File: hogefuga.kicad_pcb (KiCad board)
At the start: 2 copper layers, 95.3 x 97.6 mm, 45 parts, among them J1 MJ-4PP-9, SW1 SW_PUSH, SW10 SW_PUSH, SW11 SW_PUSH, SW12 SW_PUSH, SW13 SW_PUSH, SW14 SW_PUSH, SW15 SW_PUSH, SW16 SW_PUSH, SW17 SW_PUSH, SW18 SW_PUSH, SW19 SW_PUSH, SW2 SW_PUSH, SW20 SW_PUSH, SW3 SW_PUSH, SW4 SW_PUSH, SW5 SW_PUSH, SW6 SW_PUSH, SW7 SW_PUSH, SW8 SW_PUSH, SW9 SW_PUSH, U1 ProMicro

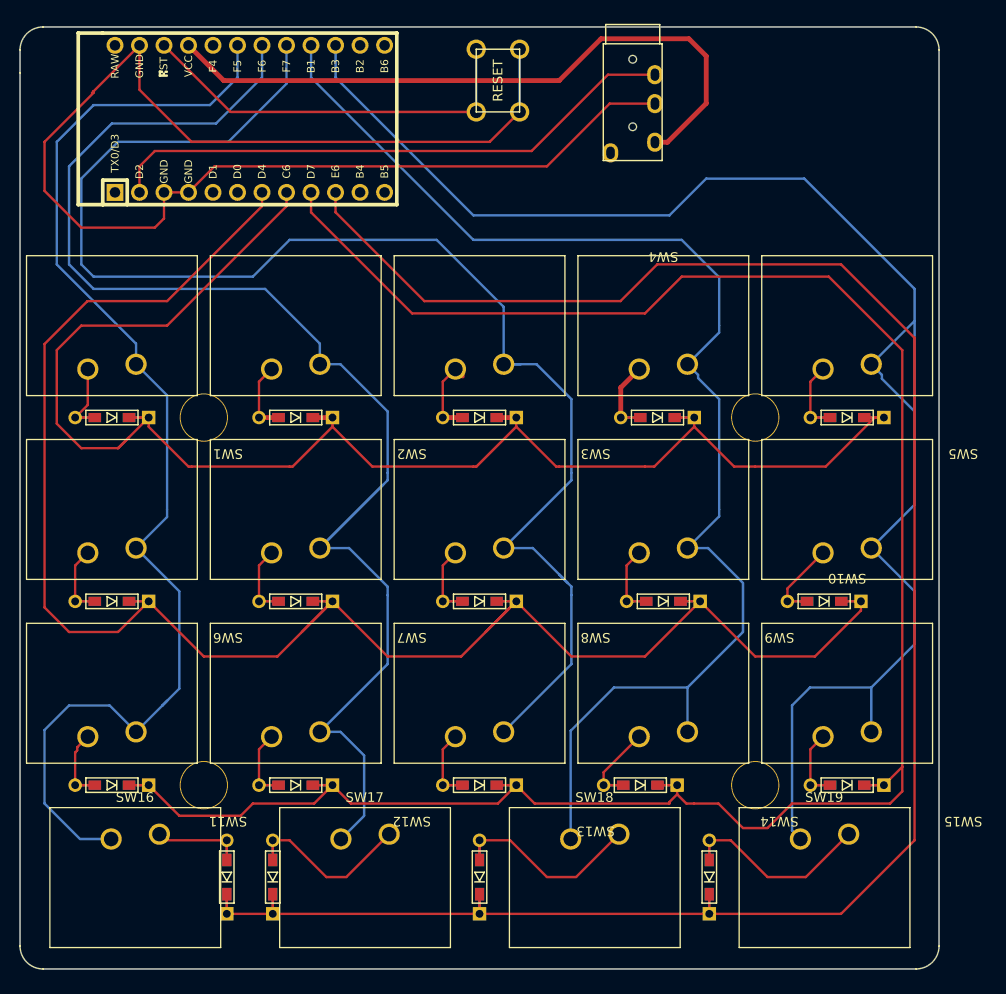
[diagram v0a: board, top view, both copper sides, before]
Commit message: GND塗りつぶし
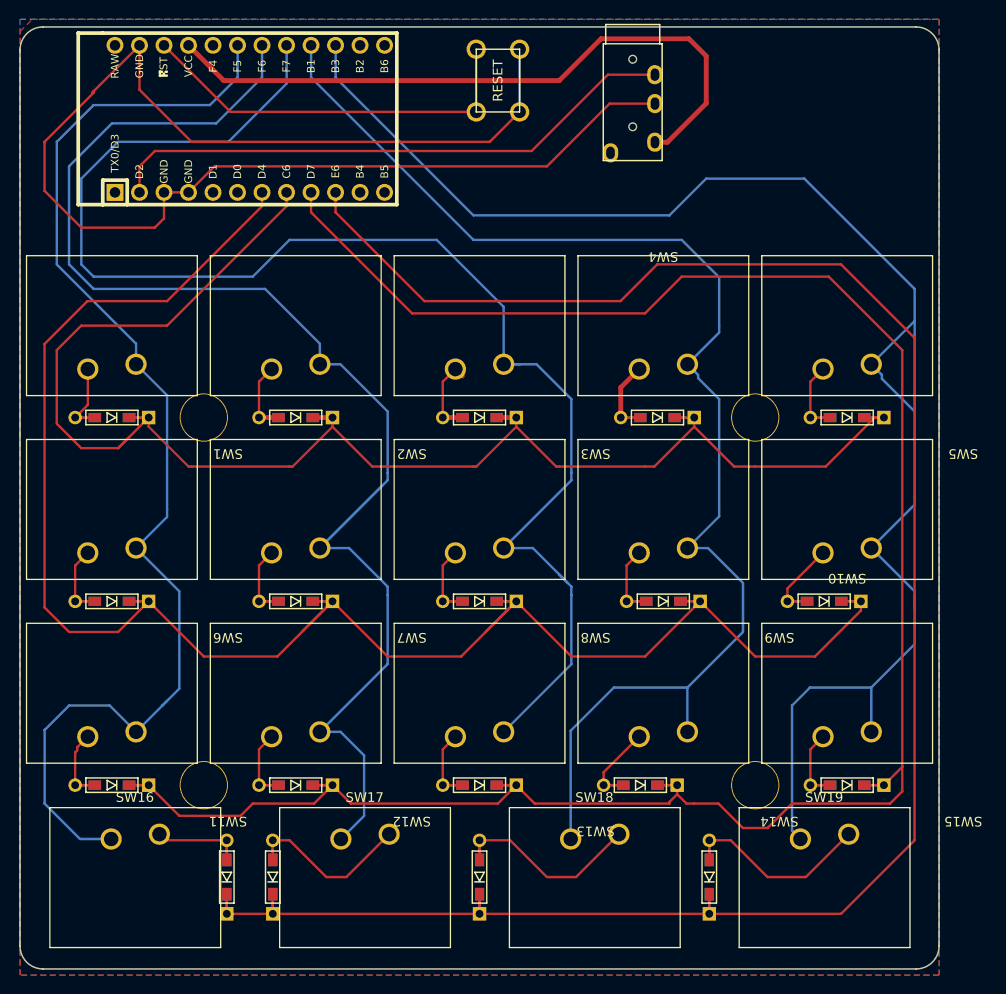
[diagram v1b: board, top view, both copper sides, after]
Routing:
- added copper zone on B.Cu, net GND
- added copper zone on F.Cu, net GND
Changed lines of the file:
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@@
   (page A4)
   (layers
-    (0 F.Cu signal)
+    (0 F.Cu signal hide)
     (31 B.Cu signal)
     (32 B.Adhes user)
@@
   (segment (start 110.1725 39.0525) (end 118.085 31.14) (width 0.25) (layer F.Cu) (net 40))
   (segment (start 69.5325 40.64) (end 71.12 39.0525) (width 0.25) (layer F.Cu) (net 40))
+  (zone (net 30) (net_name GND) (layer F.Cu) (hatch edge 0.508)
+    (connect_pads (clearance 0.508))
+    (min_thickness 0.254)
+    (fill yes (arc_segments 16) (thermal_gap 0.508) (thermal_bridge_width 0.508))
+    (polygon
+      (pts
+        (xy 152.4 25.4) (xy 152.4 124.46) (xy 57.15 124.46) (xy 57.15 26.67) (xy 58.42 25.4)
+      )
+    )
+  )
+  (zone (net 30) (net_name GND) (layer B.Cu) (hatch edge 0.508)
+    (connect_pads (clearance 0.508))
+    (min_thickness 0.254)
+    (fill yes (arc_segments 16) (thermal_gap 0.508) (thermal_bridge_width 0.508))
+    (polygon
+      (pts
+        (xy 152.4 25.4) (xy 152.4 124.46) (xy 57.15 124.46) (xy 57.15 25.4)
+      )
+    )
+  )
 )
